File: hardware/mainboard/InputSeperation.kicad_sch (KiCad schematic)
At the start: 5 parts, among them U2 LM397

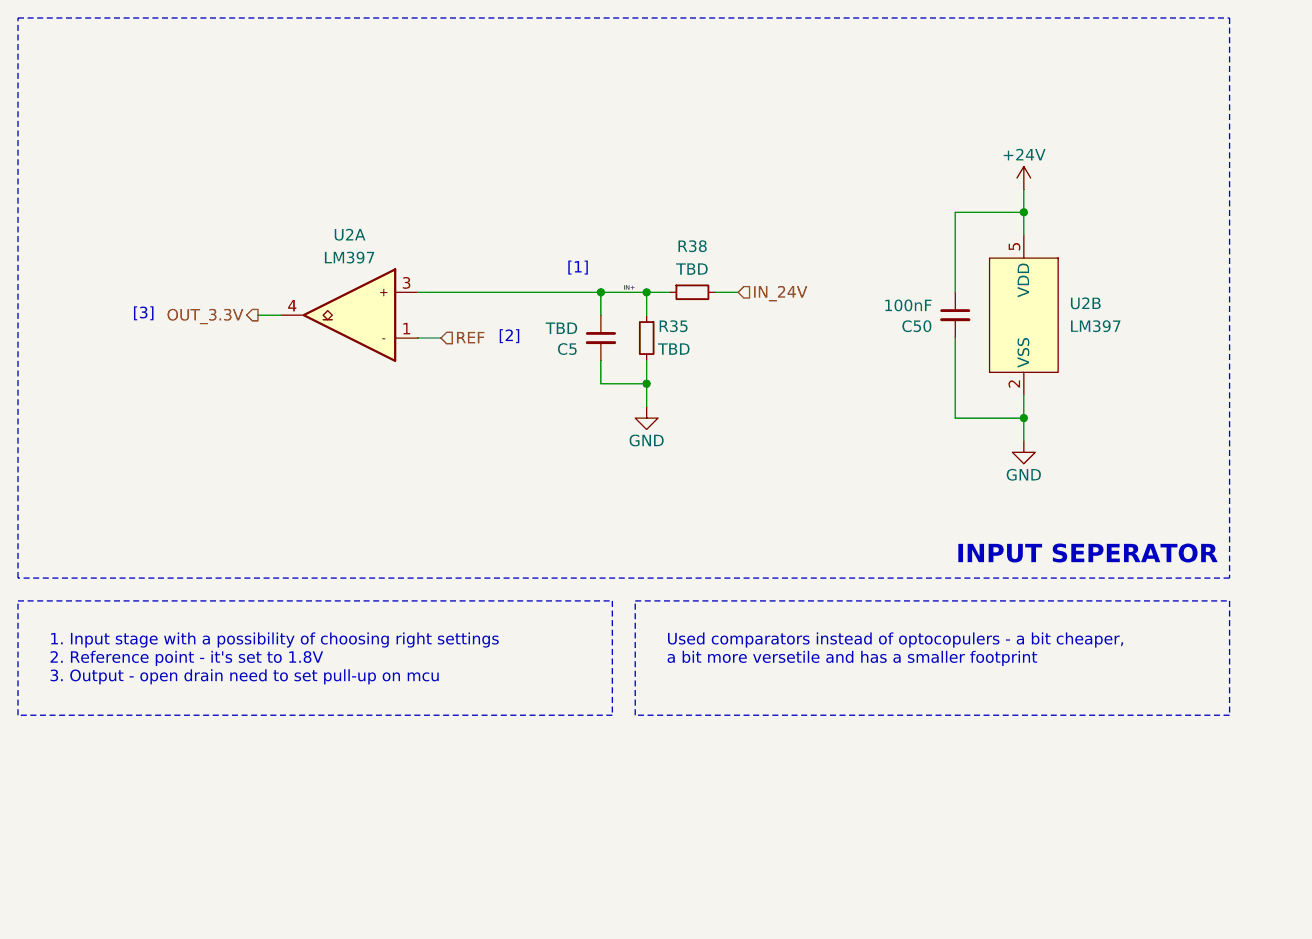
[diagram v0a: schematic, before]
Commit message: schematic?
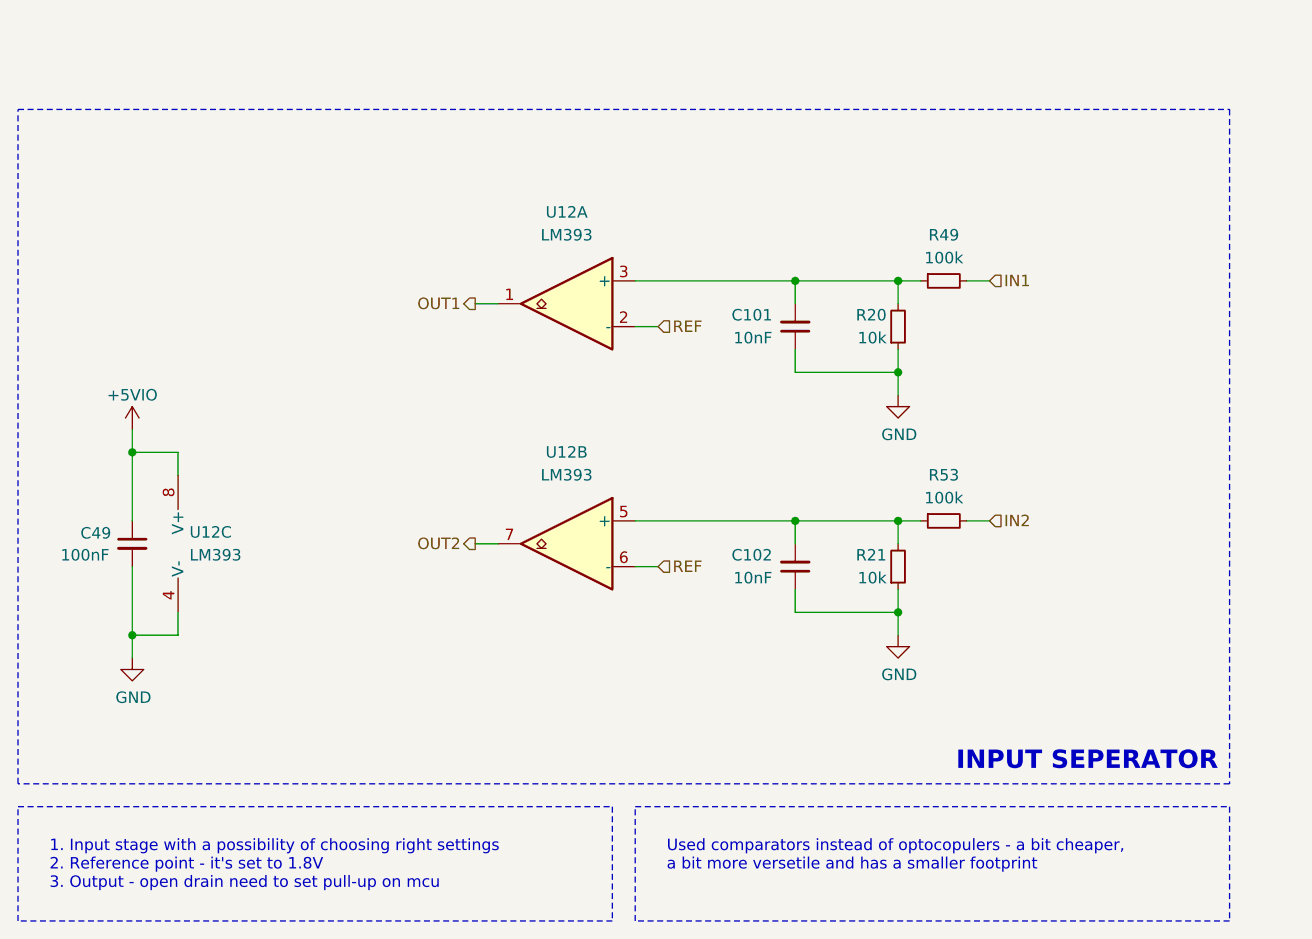
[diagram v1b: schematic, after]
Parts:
- removed C5: TBD, Capacitor_SMD:C_0603_1608Metric, symbol Device:C_Small
- removed C50: 100nF, Capacitor_SMD:C_0603_1608Metric, symbol Device:C_Small
- removed R35, R38: TBD, Resistor_SMD:R_0603_1608Metric, symbol Device:R_Small
- removed U2: LM397, Package_TO_SOT_SMD:SOT-23-5, symbol Comparator:LM397
- added C101, C102: 10nF, Capacitor_SMD:C_0603_1608Metric, symbol Device:C_Small
- added C49: 100nF, Capacitor_SMD:C_0603_1608Metric, symbol Device:C_Small
- added R20, R21: 10k, Resistor_SMD:R_0603_1608Metric, symbol Device:R_Small
- added R49, R53: 100k, Resistor_SMD:R_0603_1608Metric, symbol Device:R_Small
- added U12: LM393, Package_SO:VSSOP-8_3x3mm_P0.65mm, symbol Comparator:LM393
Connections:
- net GND: now also C101.1, C102.1, C49.2, R20.1, R21.1, U12.4 (V-)
- net REF: now also U12.2 (-), U12.6 (-)
- new net: C101.2, R20.2, R49.1, U12.3 (+)
- new net: C102.2, R21.2, R53.1, U12.5 (+)
- new net +5VIO: C49.1, U12.8 (V+)
- new net IN1: R49.2
- new net IN2: R53.2
- new net OUT1: U12.1
- new net OUT2: U12.7
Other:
- note removed: "[1]"
- note removed: "[2]"
- note removed: "[3]"
